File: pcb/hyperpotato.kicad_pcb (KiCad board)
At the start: 2 copper layers, 117 x 88.3 mm, 46 parts, among them J1 Conn_01x02_Socket, J2 Conn_01x03_Pin, Q1 AO3401A, SW1 SW_Push_45deg, SW10 SW_Push_45deg, SW11 SW_Push_45deg, SW12 SW_Push_45deg, SW13 SW_Push_45deg, SW14 SW_SPDT, SW15 SW_Push, SW2 SW_Push_45deg, SW3 SW_Push_45deg, SW4 SW_Push_45deg, SW5 SW_Push_45deg, SW6 SW_Push_45deg, SW7 SW_Push_45deg, SW8 SW_Push_45deg, SW9 SW_Push_45deg, U1 Seeeduino Xiao nRF52840, U2 SK8707-01-SENSOR, U3 SK8707-01, U4 DRV2605LDGS, U5 74HC595

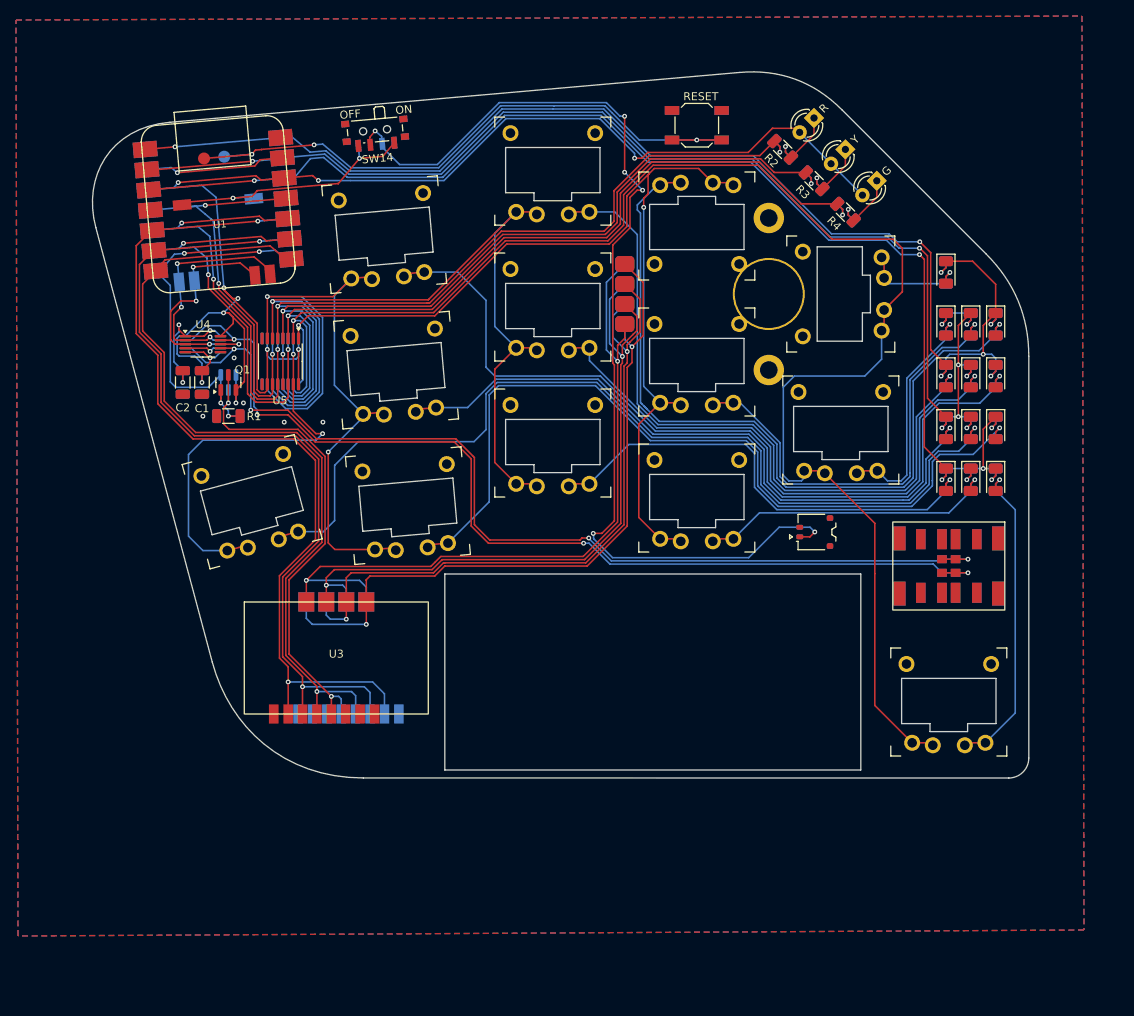
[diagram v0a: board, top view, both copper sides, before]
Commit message: Almost done!
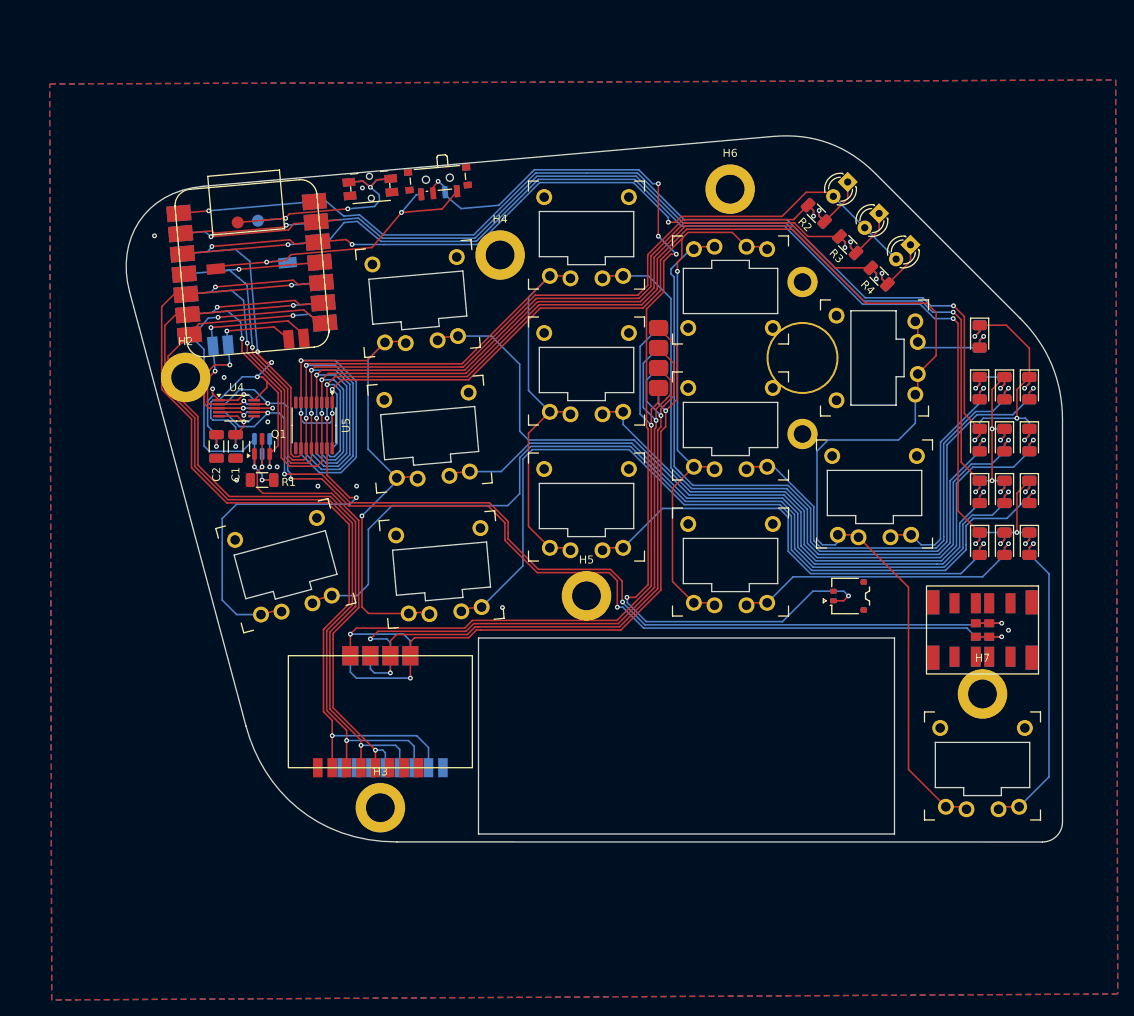
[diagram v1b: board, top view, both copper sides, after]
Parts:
- added H2: MountingHole, hyperpotato:MountingHole, F.Cu at (148.2, 101.7)
- added H3: MountingHole, hyperpotato:MountingHole, F.Cu at (172.5, 155.5)
- added H4: MountingHole, hyperpotato:MountingHole, F.Cu at (187.5, 86.4)
- added H5: MountingHole, hyperpotato:MountingHole, F.Cu at (198.3, 129.0)
- added H6: MountingHole, hyperpotato:MountingHole, F.Cu at (216.2, 78.2)
- added H7: MountingHole, hyperpotato:MountingHole, F.Cu at (247.8, 141.3)
- C1, C2: footprint ssbb_parts_reversible:C_1206_3216Metric_reversible -> hyperpotato:C_1206_3216Metric_reversible
- D1, D10, D11, D12, D13, D2, D3, D4, D5, D6, D7, D8, D9: footprint ssbb_parts_reversible:D_1206_3216Metric_reversible -> hyperpotato:D_1206_3216Metric_reversible
- H1: footprint ssbb_parts:TP_Lenovo_T460S_Sensor -> hyperpotato:TP_Lenovo_T460S_Sensor
- J1: footprint ssbb_parts_reversible:Molex_Pico-EZmate_78171-0002_1x02-1MP_P1.20mm_Vertical_reversible -> hyperpotato:Molex_Pico-EZmate_78171-0002_1x02-1MP_P1.20mm_Vertical_reversible
- J2: footprint ssbb_parts:ELV1411A_reversible -> hyperpotato:ELV1411A_reversible
- R1, R2, R3, R4: footprint ssbb_parts_reversible:R_1206_3216Metric_reversible -> hyperpotato:R_1206_3216Metric_reversible
- SW14: footprint ssbb_parts_reversible:SW_SPDT_PCM12_reversible -> hyperpotato:SW_SPDT_PCM12_reversible
- SW15: footprint ssbb_parts:SW_SPST_SKQG_WithStem_reversible -> hyperpotato:Panasonic_EVQPUL_EVQPUC_reversible
- U1: footprint hyperpotato:XIAO-nRF52840-Sense-14P-2.54-21X17.8MM_reversible -> hyperpotato:Seed_Studio_XIAO_nRF52840_reversible
- U2: footprint ssbb_parts:TP_Sensor_Connector_reversible -> hyperpotato:TP_Sensor_Connector_reversible
- U3: footprint ssbb_parts:TP_Sprintek_SK8707-01_reversible -> hyperpotato:TP_Sprintek_SK8707-01_reversible
- U4: footprint ssbb_parts_reversible:VSSOP-10_3x3mm_P0.5mm_reversible -> hyperpotato:VSSOP-10_3x3mm_P0.5mm_reversible
- U5: footprint ssbb_parts_reversible:TSSOP-16_4.4x5mm_P0.65mm_reversible -> hyperpotato:TSSOP-16_4.4x5mm_P0.65mm_reversible
- moved SW15 41.5 mm to (171.2, 78.0), turned to 5 degrees
- moved SW14 9.91 mm to (179.7, 77.2)
- moved D15 9.04 mm to (234.8, 81.2)
- moved Q1 9.04 mm to (157.7, 110.4)
- moved SW2 9.04 mm to (198.3, 83.9)
- moved U1 9.04 mm to (156.4, 88.1)
- moved D4 9.04 mm to (247.4, 96.6)
- moved R2 9.04 mm to (227.0, 81.2)
- moved R1 9.04 mm to (157.7, 114.6)
- moved D2 9.04 mm to (247.4, 109.6)
- moved D8 9.04 mm to (250.5, 103.1)
- moved SW7 9.04 mm to (198.3, 100.9)
- moved SW9 9.04 mm to (234.3, 116.3)
- moved R3 9.04 mm to (230.9, 85.1)
- moved C2 9.04 mm to (152.0, 110.4)
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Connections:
- net +3.3V_OPTIONAL renamed +3.3V_TP
- U2 pad 1: TP_S1 -> TP_VCC
- U2 pad 2: TP_S2 -> TP_GND
- U2 pad 3: TP_S3 -> TP_Y
- U2 pad 4: TP_S4 -> TP_X
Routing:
- net TP_S1: track 93.1 -> 0.00 mm, vias 2 -> 0
- net TP_VCC: track 0.00 -> 91.3 mm, vias 0 -> 2
- net TP_S4: track 88.6 -> 0.00 mm, vias 2 -> 0
- net TP_S2: track 86.4 -> 0.00 mm, vias 2 -> 0
- net TP_X: track 0.00 -> 86.1 mm, vias 0 -> 2
- net TP_S3: track 86.0 -> 0.00 mm, vias 2 -> 0
- net TP_Y: track 0.00 -> 83.7 mm, vias 0 -> 2
- net TP_GND: track 0.00 -> 81.9 mm, vias 0 -> 2
- net RESET: track 80.7 -> 36.0 mm
- net +BATT: track 32.3 -> 38.7 mm
- net VBAT: track 129.2 -> 123.3 mm
- net GND: track 31.2 -> 34.0 mm, vias 9 -> 14
- net Net-(J2-Pin_2): track 124.3 -> 121.9 mm
- net +3.3V_TP: track 61.9 -> 60.0 mm
- net Net-(J2-Pin_1): track 126.3 -> 124.6 mm
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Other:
- board text removed: "OFF"
- board text removed: "ON"
- board text removed: "RESET"
